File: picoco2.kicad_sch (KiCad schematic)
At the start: 19 parts, among them J1 Conn_01x03_Female, Q1 Q_NMOS_GDS, SW1 SW_Push, SW2 SW_Push, U1 PicoW, U2 scd30, U3 ssd1306

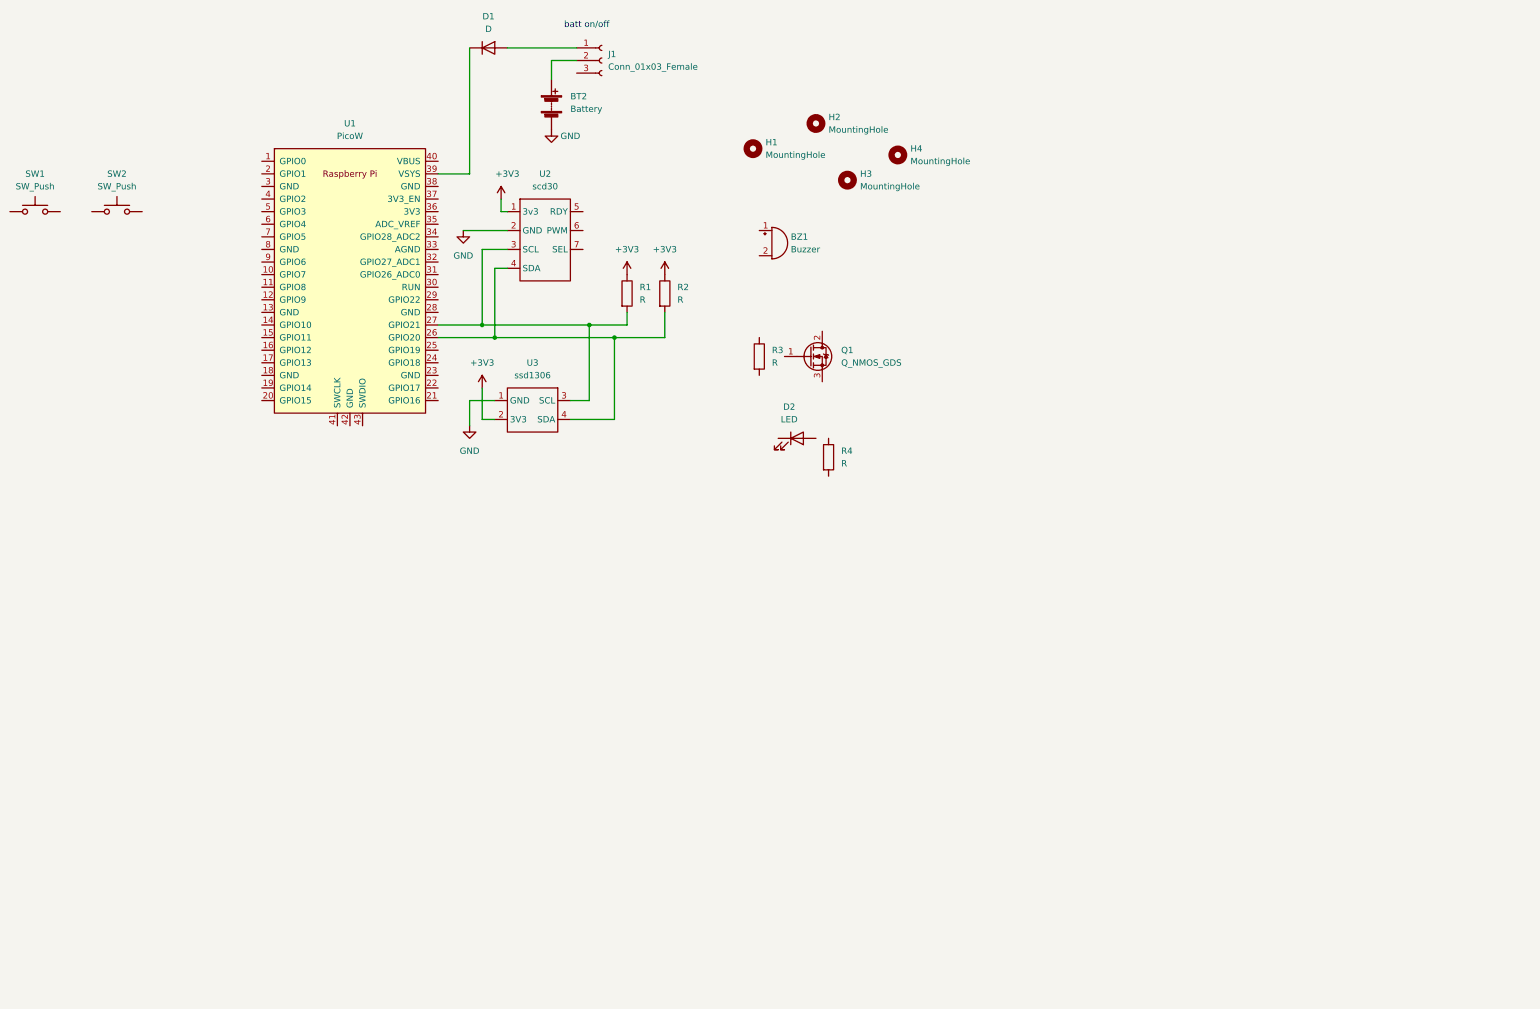
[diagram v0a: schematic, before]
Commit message: update
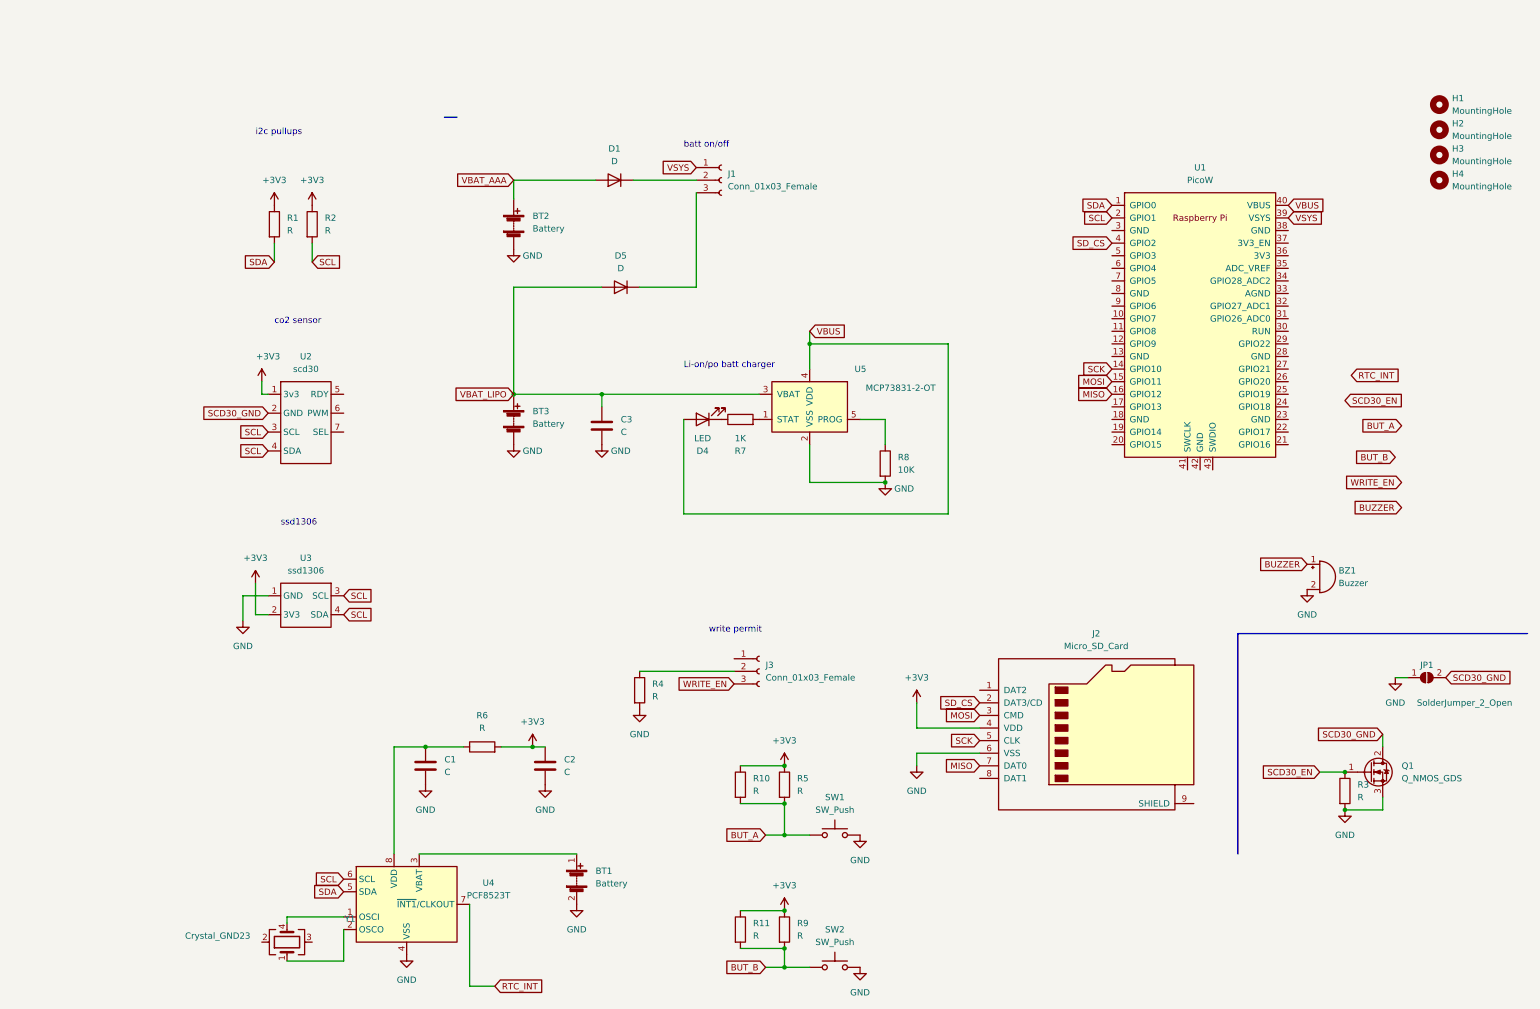
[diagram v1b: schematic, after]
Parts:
- removed D2: LED, LED_THT:LED_D5.0mm, symbol Device:LED
- added BT1: Battery, picoco2:CR1220-2, symbol Device:Battery
- added BT3: Battery, Connector_JST:JST_PH_S2B-PH-SM4-TB_1x02-1MP_P2.00mm_Horizontal, symbol Device:Battery
- added C1, C2, C3: C, Capacitor_SMD:C_0603_1608Metric_Pad1.08x0.95mm_HandSolder, symbol Device:C
- added D4: LED, LED_SMD:LED_0603_1608Metric_Pad1.05x0.95mm_HandSolder, symbol Device:LED
- added D5: D, Diode_SMD:D_SOD-123F, symbol Device:D
- added J2: Micro_SD_Card, picoco2:DM3D-SF_outline, symbol Connector:Micro_SD_Card
- added J3: Conn_01x03_Female, Connector_PinSocket_2.54mm:PinSocket_1x03_P2.54mm_Vertical, symbol Connector:Conn_01x03_Female
- added JP1: SolderJumper_2_Open, Jumper:SolderJumper-2_P1.3mm_Open_Pad1.0x1.5mm, symbol Jumper:SolderJumper_2_Open
- added R10, R11: R, Resistor_THT:R_Axial_DIN0204_L3.6mm_D1.6mm_P7.62mm_Horizontal, symbol Device:R
- added R5, R6, R9: R, Resistor_SMD:R_0603_1608Metric_Pad0.98x0.95mm_HandSolder, symbol Device:R
- added R7: 1K, Resistor_SMD:R_0603_1608Metric_Pad0.98x0.95mm_HandSolder, symbol Device:R
- added R8: 10K, Resistor_SMD:R_0603_1608Metric_Pad0.98x0.95mm_HandSolder, symbol Device:R
- added U4: PCF8523T, Package_SO:SOIC-8_3.9x4.9mm_P1.27mm, symbol Timer_RTC:PCF8523T
- added U5: MCP73831-2-OT, Package_TO_SOT_SMD:SOT-23-5, symbol Battery_Management:MCP73831-2-OT
- added Y1: Crystal_GND23, Crystal:Crystal_SMD_Abracon_ABS25-4Pin_8.0x3.8mm, symbol Device:Crystal_GND23
- BZ1: footprint Buzzer_Beeper:Buzzer_12x9.5RM7.6 -> Buzzer_Beeper:MagneticBuzzer_Kobitone_254-EMB84Q-RO
- D1: footprint Diode_THT:D_A-405_P7.62mm_Horizontal -> Diode_SMD:D_SOD-123F
- Q1: footprint Package_TO_SOT_THT:TO-220-3_Horizontal_TabDown -> Package_TO_SOT_SMD:SOT-23
- R1, R2, R3, R4: footprint Resistor_THT:R_Axial_DIN0207_L6.3mm_D2.5mm_P7.62mm_Horizontal -> Resistor_SMD:R_0603_1608Metric_Pad0.98x0.95mm_HandSolder
- U1: footprint RPi_Pico:RPi_PicoW_SMD_TH -> RPi_Pico:RPi_PicoW_SMD
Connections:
- net +3V3: now also C2.1, J2.4 (VDD), R10.1, R11.1, R5.1, R6.2, R9.1
- net GND: now also BZ1.2 (+), Q1.3 (S), R3.2, R4.2, SW1.2, SW2.2, BT1.2 (-), BT3.2 (-), C1.2, C2.2, C3.2, J2.6 (VSS), JP1.1 (A), R8.2, U4.4 (VSS), U5.2 (VSS); no longer U2.2 (GND)
- net VBAT_AAA: now reaches D1.2 (A)
- net VBAT_AAA: now also BT2.1 (+); no longer J1.1 (Pin_1)
- net at J1.2 (Pin_2): now also D1.1 (K); no longer BT2.1 (+)
- net at J1.3 (Pin_3): now also D5.1 (K)
- net SCD30_EN: now reaches Q1.1 (G)
- net SCD30_EN: now also R3.1
- net SCD30_GND: now reaches Q1.2 (D)
- net SCD30_GND: now also U2.2 (GND), JP1.2 (B)
- net SCL: now reaches R2.2, U2.4 (SDA), U3.4 (SDA)
- net SCL: now also U1.2 (GPIO1), U2.3 (SCL), U3.3 (SCL), U4.6 (SCL); no longer U1.26 (GPIO20)
- net SDA: now reaches U1.1 (GPIO0)
- net SDA: now also R1.2, U4.5 (SDA)
- net SCK: now reaches U1.14 (GPIO10)
- net SCK: now also J2.5 (CLK)
- net MOSI: now reaches U1.15 (GPIO11)
- net MOSI: now also J2.3 (CMD)
- net MISO: now reaches U1.16 (GPIO12)
- net MISO: now also J2.7 (DAT0)
- net VSYS: now reaches U1.39 (VSYS)
- net VSYS: now also J1.1 (Pin_1); no longer D1.1 (K)
- net SD_CS: now reaches U1.4 (GPIO2)
- net SD_CS: now also J2.2 (DAT3/CD)
- net VBUS: now reaches U1.40 (VBUS)
- net VBUS: now also D4.2 (A), U5.4 (VDD)
- net at R4.1: now also J3.2 (Pin_2)
- net BUT_A: now reaches SW1.1
- net BUT_A: now also R10.2, R5.2
- net BUT_B: now reaches SW2.1
- net BUT_B: now also R11.2, R9.2
- net BUZZER: now reaches BZ1.1 (-)
- new net: U4.2 (OSCO), Y1.1
- new net: U4.1 (OSCI), Y1.4
- new net: D4.1 (K), R7.1
- new net: R7.2, U5.1 (STAT)
- new net: BT1.1 (+), U4.3 (VBAT)
- new net: C1.1, R6.1, U4.8 (VDD)
- new net: R8.1, U5.5 (PROG)
- new net RTC_INT: U4.7 (~{INT1}/CLKOUT)
- new net VBAT_LIPO: BT3.1 (+), C3.1, D5.2 (A), U5.3 (VBAT)
- new net WRITE_EN: J3.3 (Pin_3)
- now unconnected: U1.27 (GPIO21)
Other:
- note added: "Li-on/po batt charger"
- note added: "co2 sensor"
- note added: "i2c pullups"
- note added: "ssd1306"
- note added: "write permit"
- moved on the sheet: BT2, BZ1, D1, H1, H2, H3, H4, J1, Q1, R1, R2, R3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
